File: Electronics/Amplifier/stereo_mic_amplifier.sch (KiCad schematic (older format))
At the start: 26 parts, among them P1 mic_L, P2 mic_R, P3 batt, P4 CONN_01X03, U1 TL072

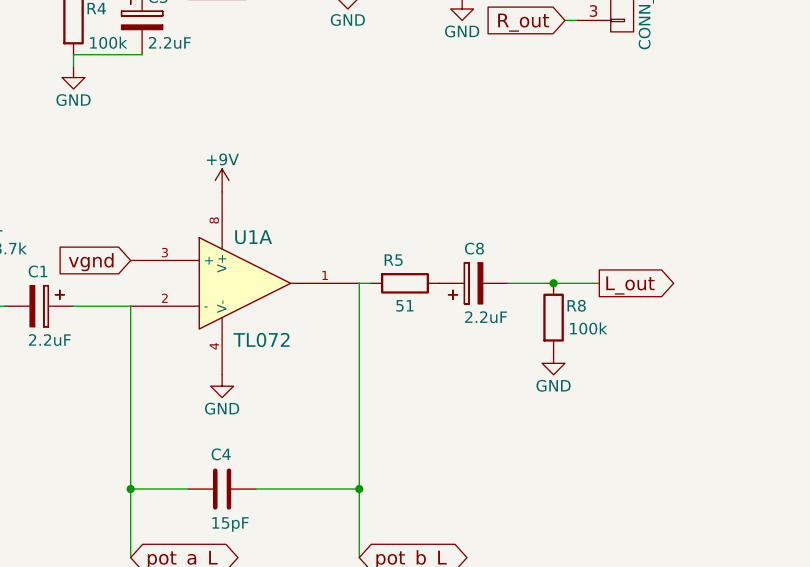
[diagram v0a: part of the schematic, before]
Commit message: Layout progress
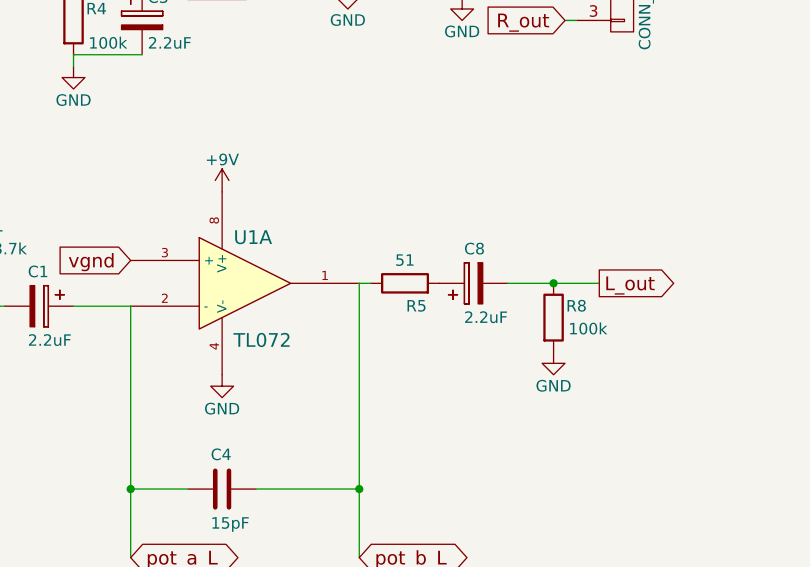
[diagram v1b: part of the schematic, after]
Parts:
- R5, R6, R8, R9: footprint Resistors_ThroughHole:Resistor_Horizontal_RM10mm -> Resistors_ThroughHole:Resistor_Vertical_RM5mm
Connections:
- net pot_b_L: now also R5.1; no longer R5.2
- net at C8.1: now also R5.2; no longer R5.1
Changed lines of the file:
@@
 LIBS:valves
 LIBS:mic_amp
+LIBS:stereo_mic_amplifier-cache
 EELAYER 25 0
 EELAYER END
@@
 F 0 "R5" V 3450 3450 50  0000 C CNN
 F 1 "51" V 3650 3500 50  0000 C CNN
-F 2 "Resistors_ThroughHole:Resistor_Horizontal_RM10mm" V 3480 3500 30  0001 C CNN
+F 2 "Resistors_ThroughHole:Resistor_Vertical_RM5mm" V 3480 3500 30  0001 C CNN
 F 3 "" H 3550 3500 30  0000 C CNN
 	1    3550 3500
-	0    1    1    0
+	0    -1   -1   0
 $EndComp
 $Comp
@@
 F 0 "R8" H 4300 3700 50  0000 C CNN
 F 1 "100k" H 4350 3600 50  0000 C CNN
-F 2 "Resistors_ThroughHole:Resistor_Horizontal_RM10mm" V 4130 3650 30  0001 C CNN
+F 2 "Resistors_ThroughHole:Resistor_Vertical_RM5mm" V 4130 3650 30  0001 C CNN
 F 3 "" H 4200 3650 30  0000 C CNN
 	1    4200 3650
@@
 F 0 "R6" V 3450 5400 50  0000 C CNN
 F 1 "51" V 3650 5450 50  0000 C CNN
-F 2 "Resistors_ThroughHole:Resistor_Horizontal_RM10mm" V 3480 5450 30  0001 C CNN
+F 2 "Resistors_ThroughHole:Resistor_Vertical_RM5mm" V 3480 5450 30  0001 C CNN
 F 3 "" H 3550 5450 30  0000 C CNN
 	1    3550 5450
@@
 F 0 "R9" H 4300 5650 50  0000 C CNN
 F 1 "100k" H 4350 5550 50  0000 C CNN
-F 2 "Resistors_ThroughHole:Resistor_Horizontal_RM10mm" V 4130 5600 30  0001 C CNN
+F 2 "Resistors_ThroughHole:Resistor_Vertical_RM5mm" V 4130 5600 30  0001 C CNN
 F 3 "" H 4200 5600 30  0000 C CNN
 	1    4200 5600
